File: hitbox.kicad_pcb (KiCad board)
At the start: 2 copper layers, 5 x 5 mm, 19 parts, among them U1 ER_OLEDM0.91_1x-I2C

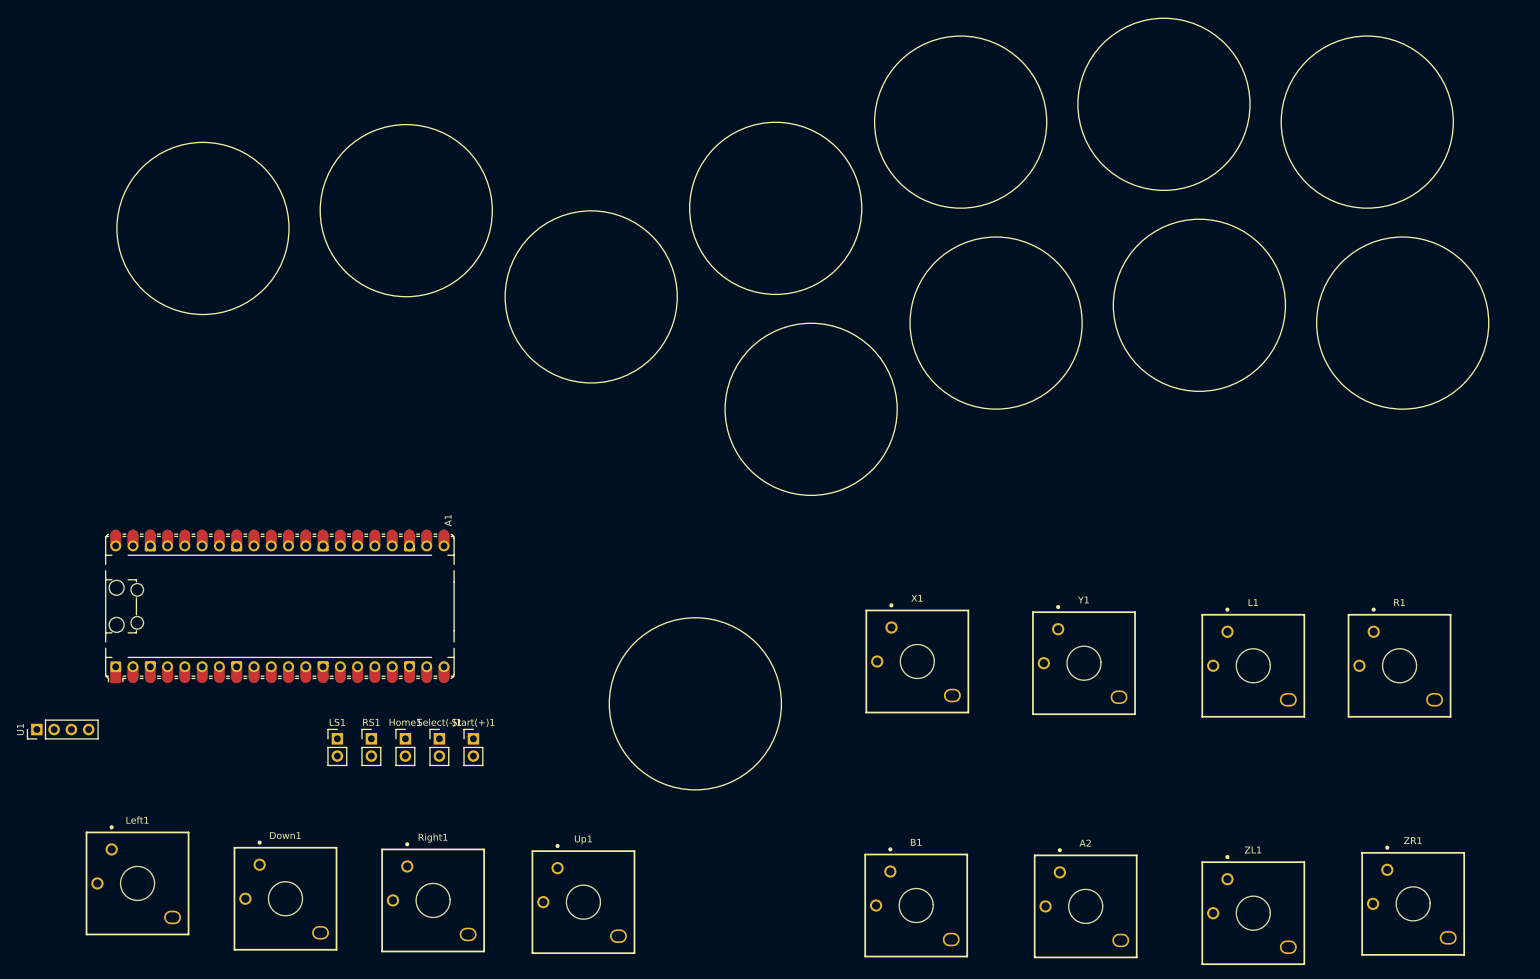
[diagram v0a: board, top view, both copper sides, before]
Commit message: 邊框與零件位置
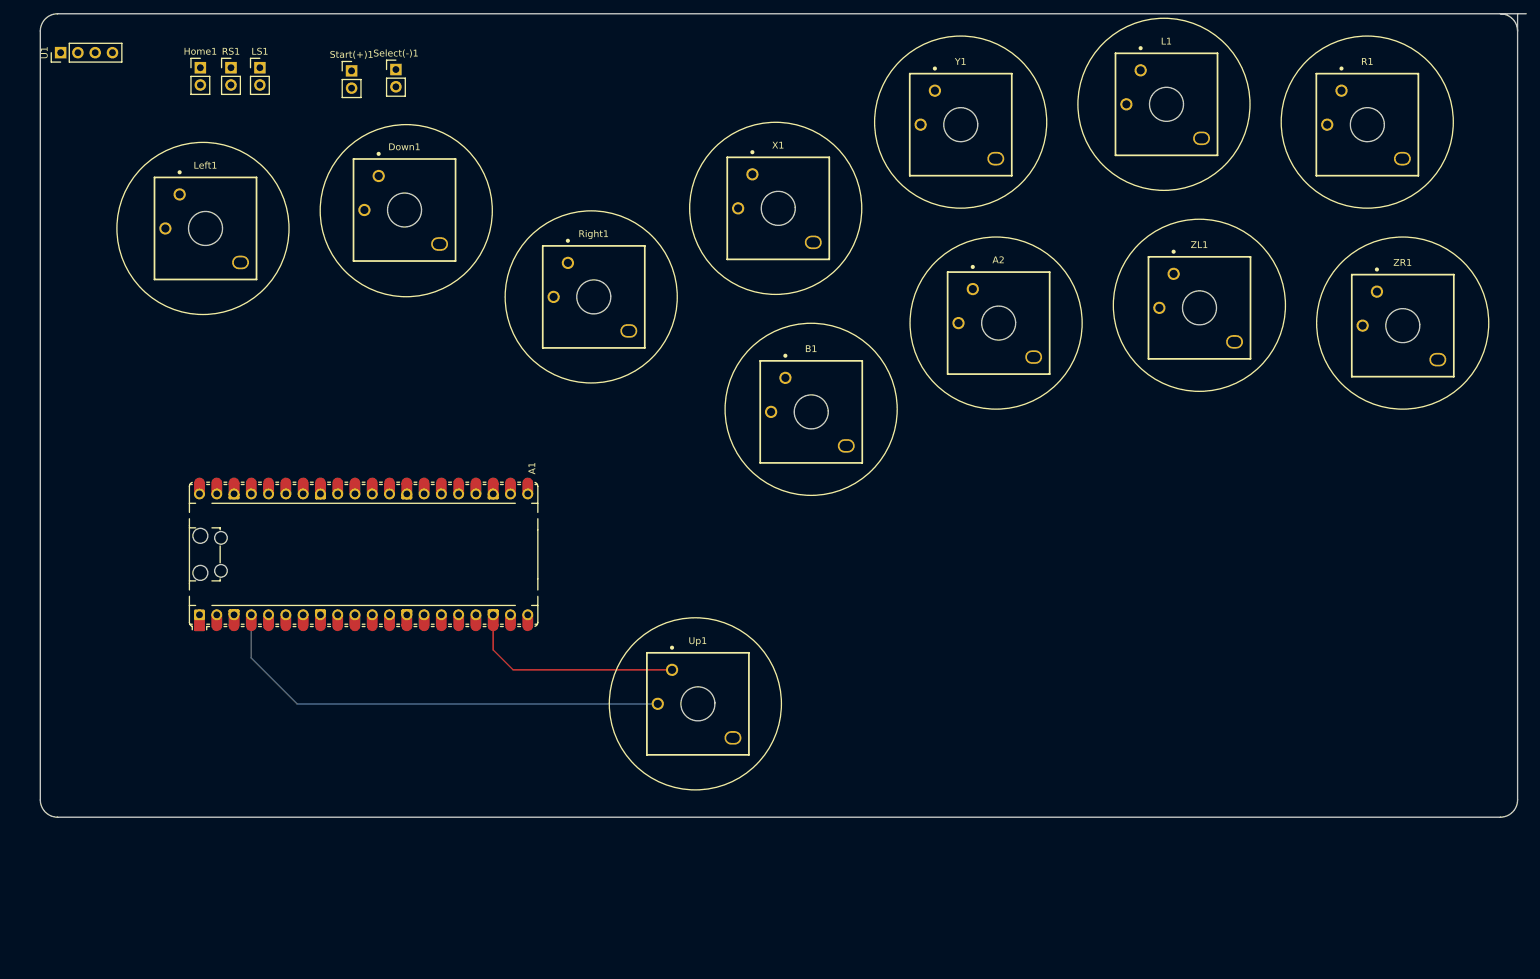
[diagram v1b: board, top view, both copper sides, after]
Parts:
- moved Home1 103.2 mm to (37.5, 25.7)
- moved Down1 102.8 mm to (67.1, 46.6)
- moved RS1 100.8 mm to (42.0, 25.7)
- moved Start(+)1 99.8 mm to (59.7, 26.2)
- moved U1 99.6 mm to (17.0, 23.5)
- moved LS1 99.3 mm to (46.2, 25.7)
- moved Select(-)1 98.6 mm to (66.2, 26.0)
- moved Left1 96.8 mm to (37.9, 49.3)
- moved Right1 91.8 mm to (95.0, 59.4)
- moved ZL1 89.3 mm to (184.0, 61.0)
- moved A2 86.7 mm to (154.5, 63.2)
- moved ZR1 85.0 mm to (213.9, 63.6)
- moved L1 83.5 mm to (179.2, 31.1)
- moved Y1 81.2 mm to (148.9, 34.1)
- moved R1 79.7 mm to (208.7, 34.1)
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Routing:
- net Net-(A1-GPIO2): track 0.00 -> 68.9 mm
- net Net-(U1-GND): track 0.00 -> 31.9 mm
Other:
- board size 5 x 5 mm -> 218.4 x 118.1 mm
